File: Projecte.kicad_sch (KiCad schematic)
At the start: 48 parts, among them K1 A161CS12VDC.64, Q1 IRLZ34N, Q2 BC107, Q3 IRLZ34N, Q4 IRLZ34N, Q5 IRLZ34N, Q6 IRLZ34N, Q7 IRLZ34N, U1 PIC18F448-IP, U2 LM358, U3 R-786.5-0.5, U4 MCP2551-I-P, U5 AMS1117-3.3, U6 TXB0108PW, U7 LM7805_TO220, Y1 Crystal

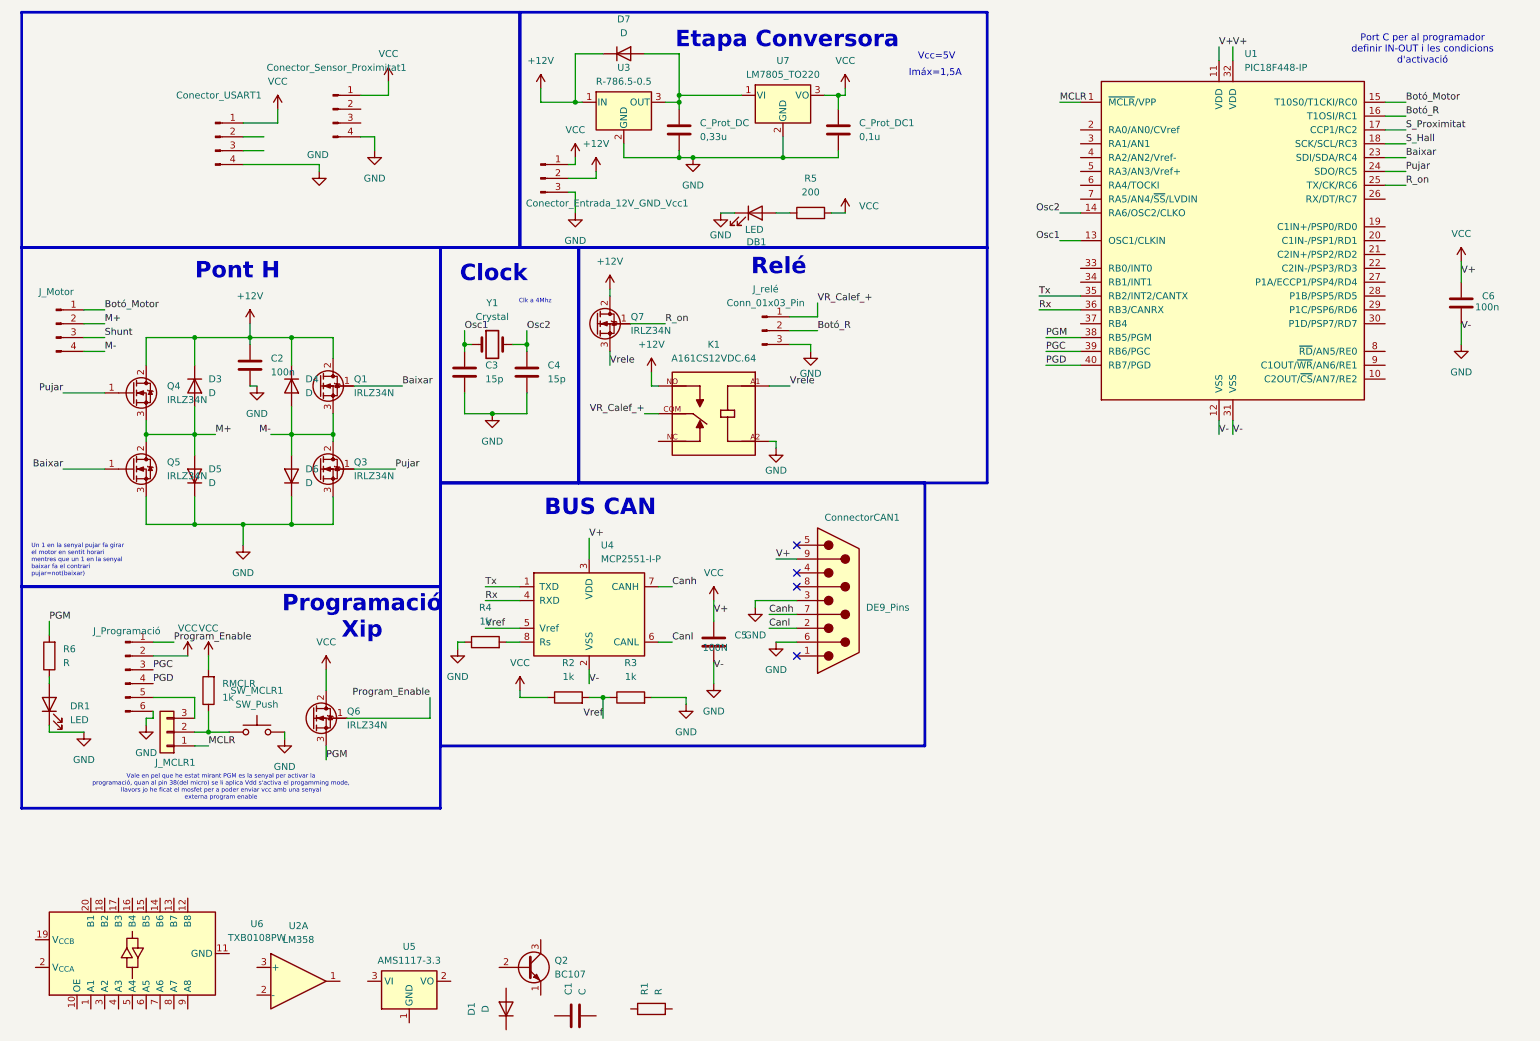
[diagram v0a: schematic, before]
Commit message: Update Proyecto.kicad_sch
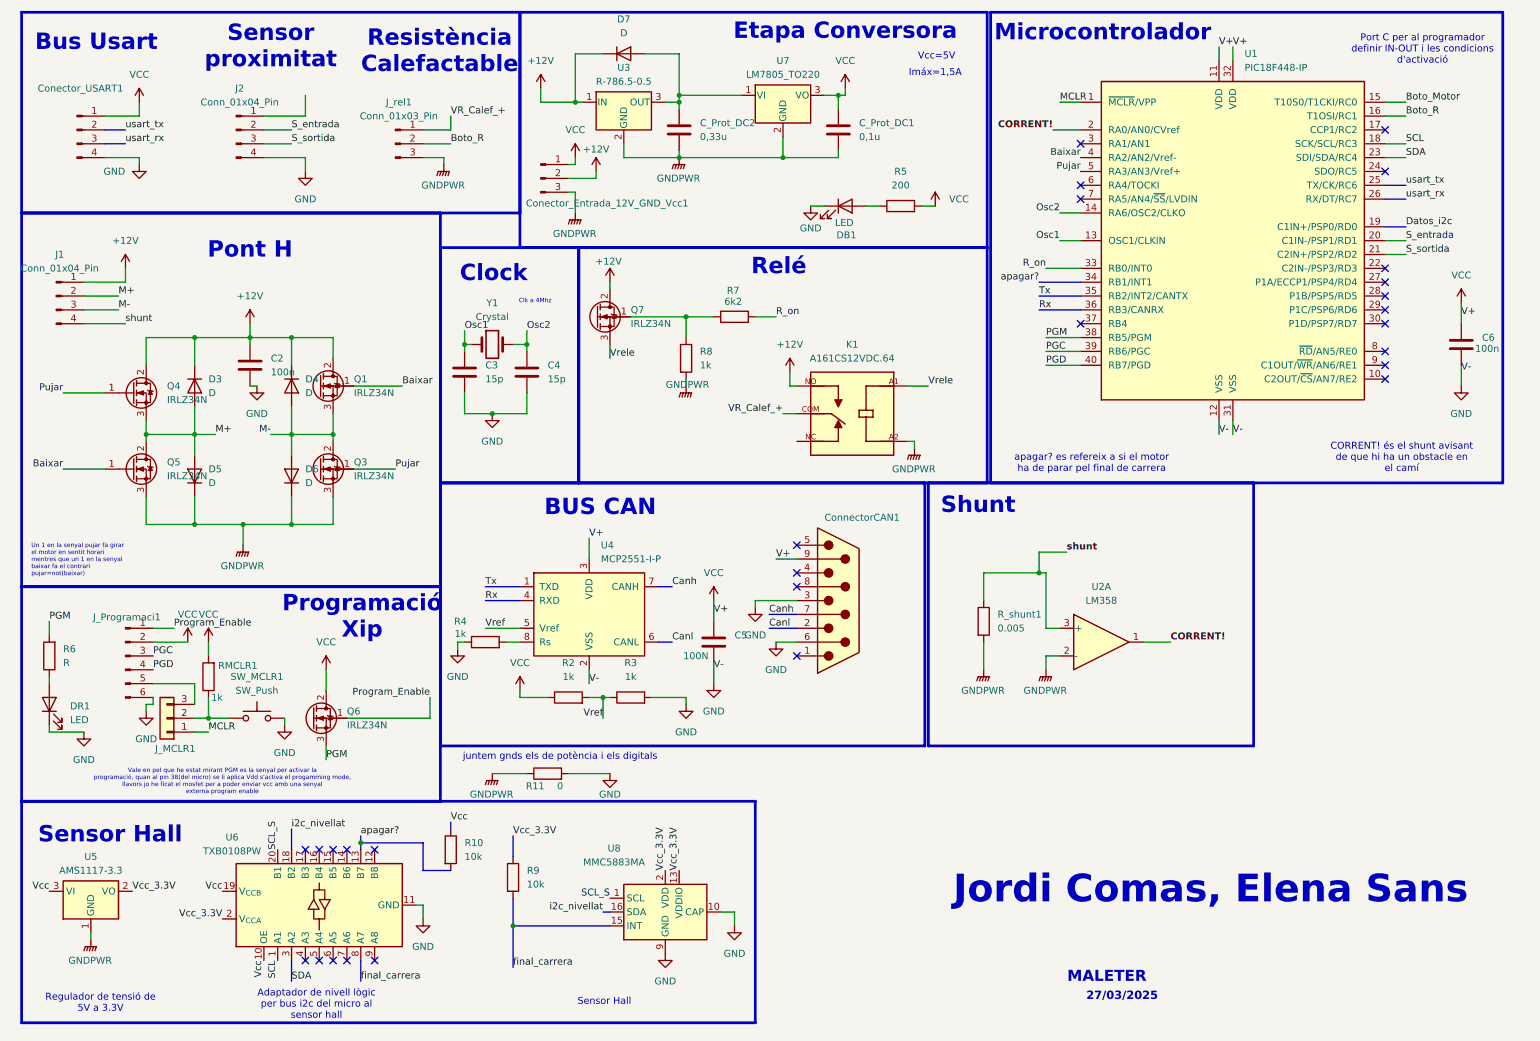
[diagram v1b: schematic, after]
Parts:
- removed C1: C, symbol Device:C
- removed Conector_Sensor_Proximitat1, J_Motor: Conn_01x04_Pin, symbol Connector:Conn_01x04_Pin
- removed D1: D, symbol Device:D
- removed Q2: BC107, Package_TO_SOT_THT:TO-18-3, symbol Transistor_BJT:BC107
- removed R1: R, symbol Device:R
- added J1, J2: Conn_01x04_Pin, symbol Connector:Conn_01x04_Pin
- added R10, R9: 10k, symbol Device:R
- added R11: 0, symbol Device:R
- added R7: 6k2, symbol Device:R
- added R8: 1k, symbol Device:R
- added R_shunt1: 0.005, symbol Device:R
- added U8: MMC5883MA, Package_LGA:LGA-16_3x3mm_P0.5mm, symbol Sensor_Magnetic:MMC5883MA
- renumbered C_Prot_DC to C_Prot_DC2, J_Programació to J_Programaci1, J_relé to J_rel1, RMCLR to RMCLR1
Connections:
- net S_Hall is gone; now on net SCL: U1.18 (SCK/SCL/RC3)
- net +12V: now also J1.1 (Pin_1)
- net Baixar: now also U1.4 (RA2/AN2/Vref-); no longer U1.23 (SDI/SDA/RC4)
- net Canh: no longer ConnectorCAN1.7, U4.7 (CANH)
- net Canl: no longer ConnectorCAN1.2, U4.6 (CANL)
- net GND: now also U6.11 (GND), J2.4 (Pin_4), R11.2, U8.10 (CAP), U8.11 (GND), U8.9 (GND); no longer C_Prot_DC1.2, C_Prot_DC2.2, Conector_Entrada_12V_GND_Vcc1.3 (Pin_3), D5.1 (K), D6.1 (K), J_rel1.3 (Pin_3), K1.A2, Q3.3 (S), Q5.3 (S), U3.2 (GND), U7.2 (GND)
- net M+: now also J1.2 (Pin_2)
- net M-: now also J1.3 (Pin_3)
- net Pujar: now also U1.5 (RA3/AN3/Vref+); no longer U1.24 (SDO/RC5)
- net R_on: now also U1.33 (RB0/INT0), R7.2; no longer Q7.1 (G), U1.25 (TX/CK/RC6)
- net Rx: no longer U1.36 (RB3/CANRX), U4.4 (RXD)
- net Tx: no longer U1.35 (RB2/INT2/CANTX), U4.1 (TXD)
- net GNDPWR: now reaches U5.1 (GND)
- net GNDPWR: now also C_Prot_DC1.2, C_Prot_DC2.2, Conector_Entrada_12V_GND_Vcc1.3 (Pin_3), D5.1 (K), D6.1 (K), J_rel1.3 (Pin_3), K1.A2, Q3.3 (S), Q5.3 (S), U2.2 (-), U3.2 (GND), U7.2 (GND), R11.1, R8.2, R_shunt1.2
- net Vcc_3.3V: now reaches U5.2 (VO)
- net Vcc_3.3V: now also U6.2 (V_{CCA}), U8.13 (VDDIO), U8.2 (VDD)
- net Vcc: now reaches U5.3 (VI)
- net Vcc: now also U6.10 (OE), U6.19 (V_{CCB})
- net CORRENT!: now reaches U1.2 (RA0/AN0/CVref)
- net CORRENT!: now also U2.1
- net S_entrada: now reaches U1.20 (C1IN-/PSP1/RD1)
- net S_entrada: now also J2.2 (Pin_2)
- net S_sortida: now reaches U1.21 (C2IN+/PSP2/RD2)
- net S_sortida: now also J2.3 (Pin_3)
- net shunt: now reaches U2.3 (+)
- net shunt: now also J1.4 (Pin_4), R_shunt1.1
- net SCL: now reaches U6.1 (A1)
- net SCL_S: now reaches U6.20 (B1)
- net SCL_S: now also U8.1 (SCL)
- net Botó_Motor renamed Boto_Motor
- net Botó_R renamed Boto_R
- net S_Proximitat: no longer names the net of U1.17 (CCP1/RC2)
- new net: Q7.1 (G), R7.1, R8.1
- new net SDA: U1.23 (SDI/SDA/RC4)
- no-connect marks 4 -> 28
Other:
- note added: "27/03/2025"
- note added: "Adaptador de nivell lògic per bus i2c del micro al sensor hall"
- note added: "Bus Usart"
- note added: "CORRENT! és el shunt avisant de que hi ha un obstacle en el camí"
- note added: "Jordi Comas, Elena Sans"
- note added: "MALETER"
- note added: "Microcontrolador"
- note added: "Regulador de tensió de 5V a 3.3V"
- note added: "Resistència Calefactable"
- note added: "Sensor Hall"
- note added: "Sensor proximitat"
- note added: "Shunt"
- note added: "apagar? es refereix a si el motor ha de parar pel final de carrera"
- note added: "juntem gnds els de potència i els digitals"
- moved on the sheet: C6, Conector_USART1, DB1, J_MCLR1, J_Programaci1, J_rel1, K1, Q7, R5, RMCLR1, SW_MCLR1, U2A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
